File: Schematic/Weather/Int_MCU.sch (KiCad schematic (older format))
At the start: 9 parts, among them U1 AMS1117, U2 ESP-01v090

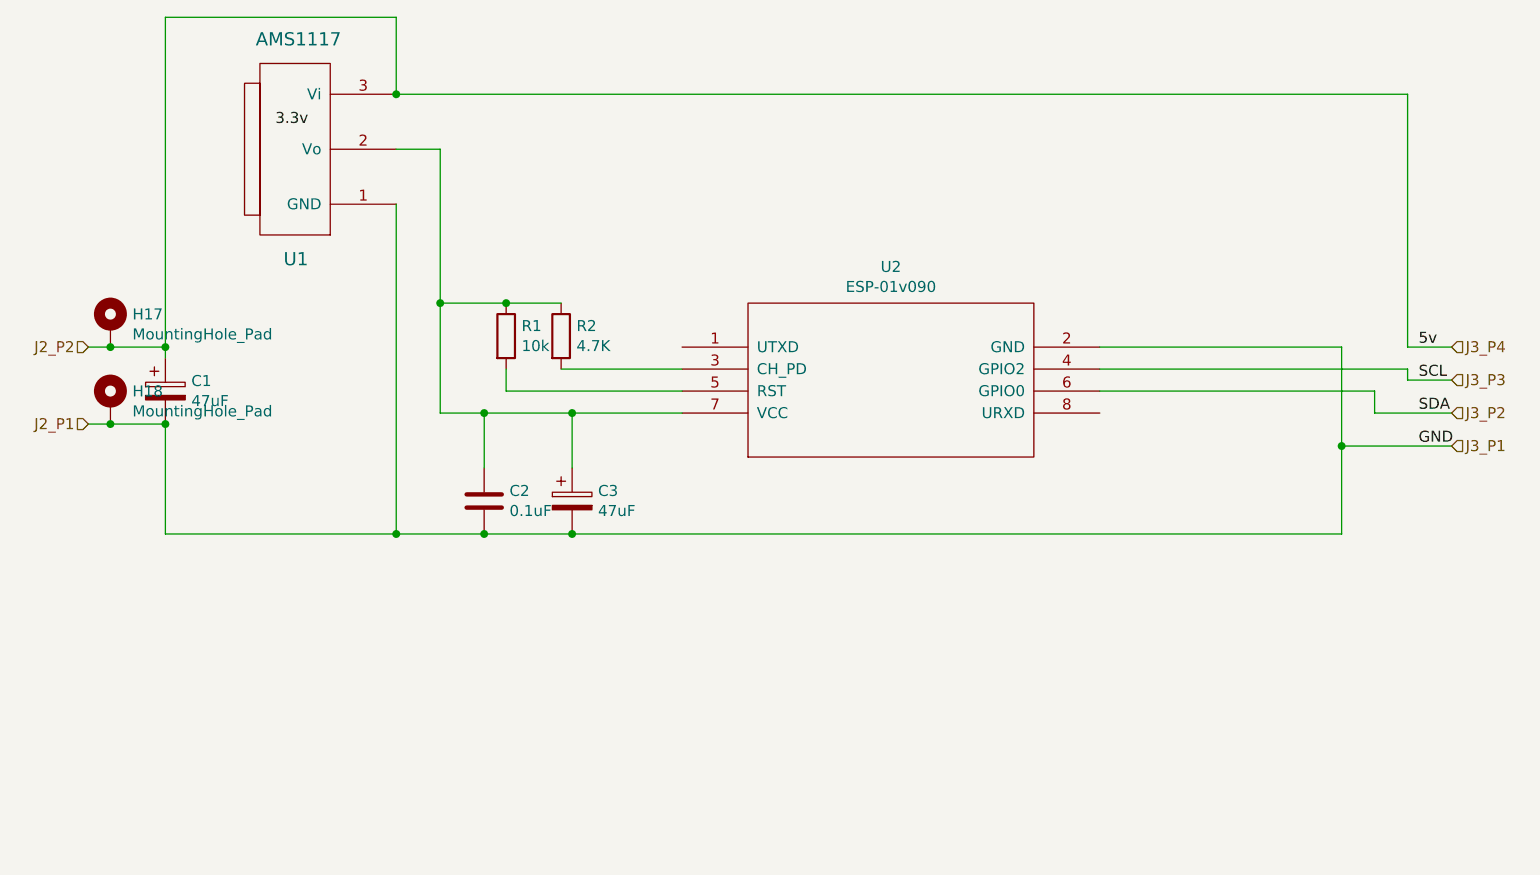
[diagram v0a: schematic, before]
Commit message: new M_Board internal
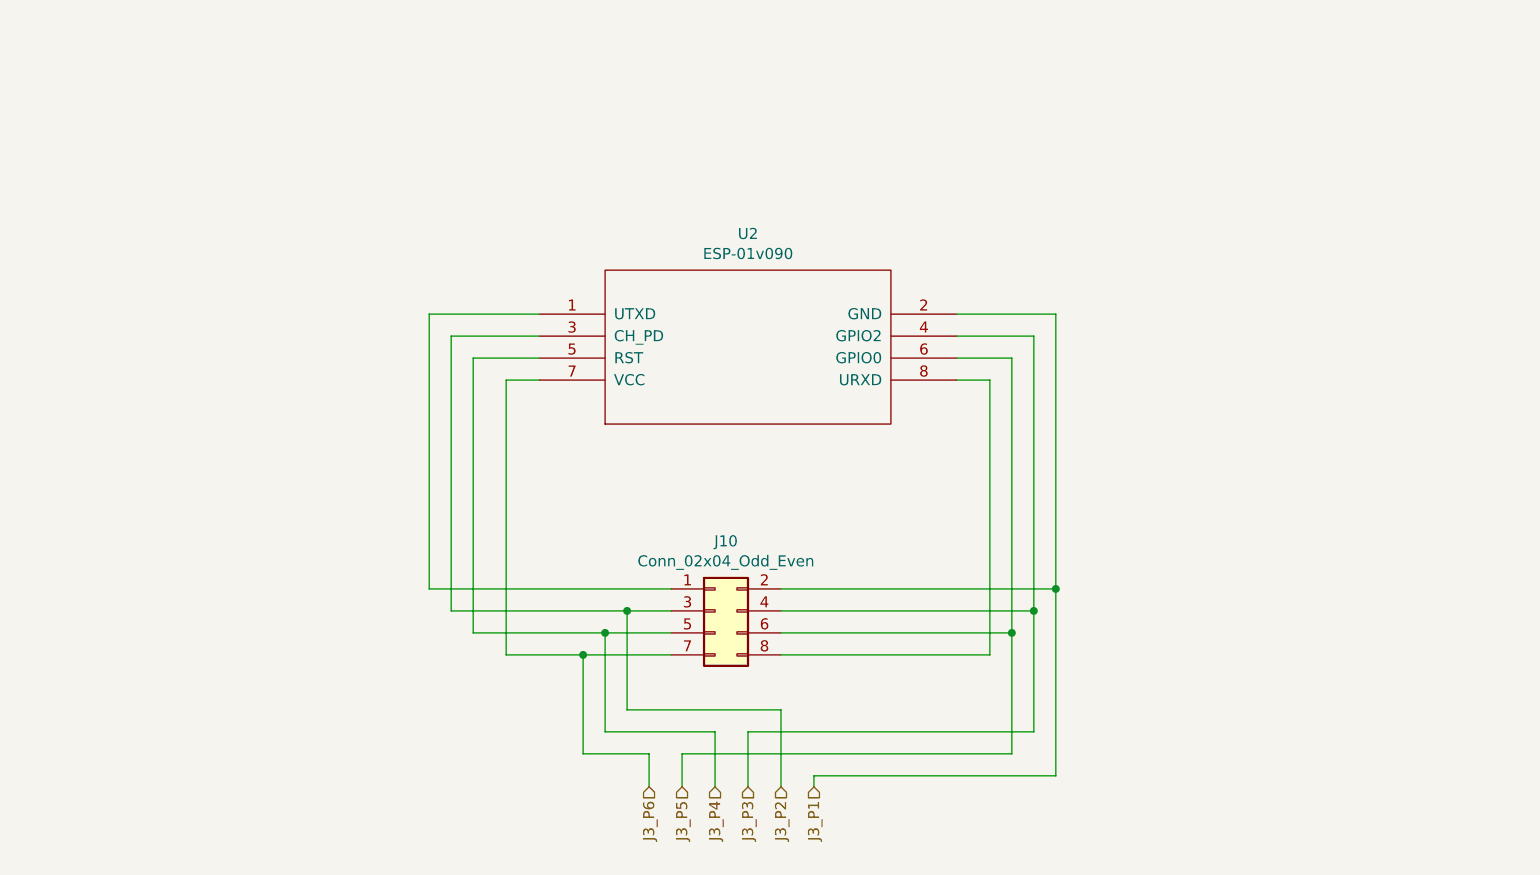
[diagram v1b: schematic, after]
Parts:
- removed C1, C3: 47uF, Capacitor_THT:CP_Radial_Tantal_D5.0mm_P2.50mm, symbol Device:CP
- removed C2: 0.1uF, Capacitor_THT:C_Disc_D3.8mm_W2.6mm_P2.50mm, symbol Device:C
- removed H17, H18: MountingHole_Pad, symbol Mechanical:MountingHole_Pad
- removed R1: 10k, Resistor_THT:R_Axial_DIN0207_L6.3mm_D2.5mm_P7.62mm_Horizontal, symbol Device:R
- removed R2: 4.7K, Resistor_THT:R_Axial_DIN0207_L6.3mm_D2.5mm_P7.62mm_Horizontal, symbol Device:R
- removed U1: AMS1117, Package_TO_SOT_SMD:SOT-223-3_TabPin2, symbol MyComponents:AMS1117
- added J10: Conn_02x04_Odd_Even, Connector_PinHeader_2.54mm:PinHeader_2x04_P2.54mm_Vertical, symbol Connector_Generic:Conn_02x04_Odd_Even
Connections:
- net J3_P2: now also U2.3 (CH_PD), J10.3 (Pin_3); no longer U2.6 (GPIO0)
- net J3_P3: now also J10.4 (Pin_4)
- net at U2.1 (UTXD): now also J10.1 (Pin_1)
- net J3_P4: now reaches U2.5 (RST)
- net J3_P4: now also J10.5 (Pin_5)
- net J3_P6: now reaches U2.7 (VCC)
- net J3_P6: now also J10.7 (Pin_7)
- net at U2.8 (URXD): now also J10.8 (Pin_8)
- net J2_P1 renamed J3_P1
- net J3_P1: now also J10.2 (Pin_2)
- new net J3_P5: J10.6 (Pin_6), U2.6 (GPIO0)
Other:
- moved on the sheet: U2
